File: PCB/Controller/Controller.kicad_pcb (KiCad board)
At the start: 2 copper layers, 100 x 90 mm, 25 parts, among them J1 Conn_01x03, J2 Conn_01x02, J3 Conn_01x08, J4 Conn_01x06, Q1 MJD6039, Q2 MJD6039, Q3 MJD6039, Q4 MJD6039, Q5 MJD6039, Q6 MJD6039, Q7 MJD6039, U1 ESP8266-01/ESP-01, U2 EK-TM4C123GXL

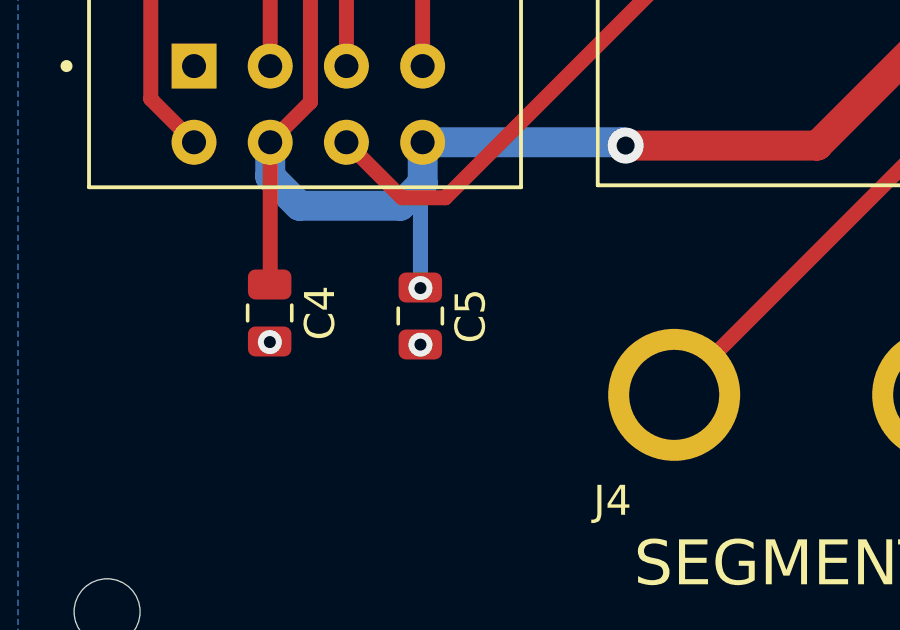
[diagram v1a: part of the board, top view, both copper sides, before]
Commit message: latest update of pcbs
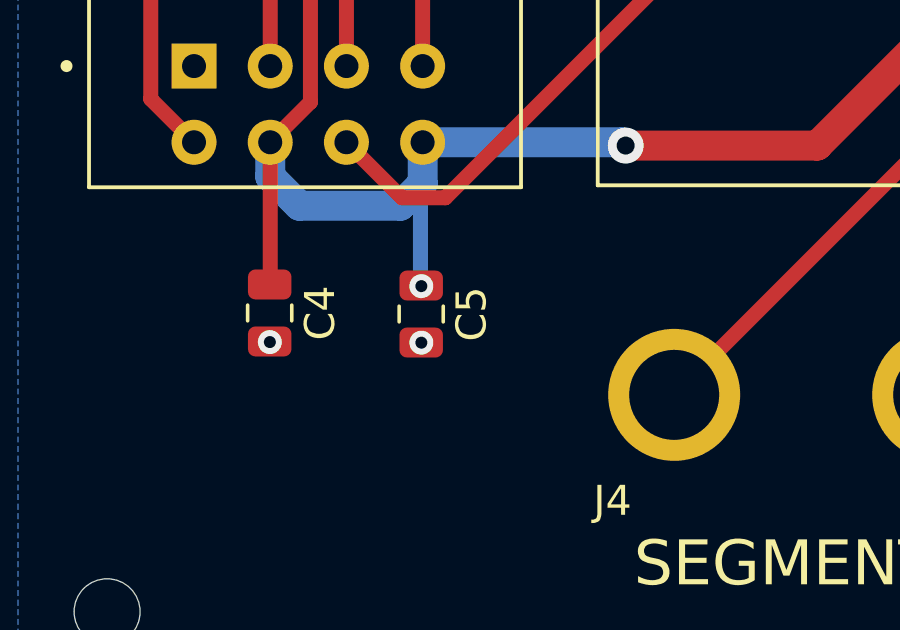
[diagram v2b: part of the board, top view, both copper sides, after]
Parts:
- moved C5 0.07 mm to (30.5, 90.1)
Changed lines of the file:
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@@
   )
   (footprint "Capacitor_SMD:C_0805_2012Metric" (layer "F.Cu")
-    (at 30.44 90.14 -90)
+    (at 30.47 90.075 -90)
     (descr "Capacitor SMD 0805 (2012 Metric), square (rectangular) end terminal, IPC_7351 nominal, (Body size source: IPC-SM-782 page 76, https://www.pcb-3d.com/wordpress/wp-content/uploads/ipc-sm-782a_amendment_1_and_2.pdf, https://docs.google.com/spreadsheets/d/1BsfQQcO9C6DZCsRaXUlFlo91Tg2WpOkGARC1WS5S8t0/edit?usp=sharing), generated with kicad-footprint-generator")
     (tags "capacitor")
@@
   (segment (start 27.315 50.225) (end 38.895 50.225) (width 1) (layer "F.Cu") (net 1))
   (via (at 47.705 80.43) (size 1.2) (drill 0.6) (layers "F.Cu" "B.Cu") (net 1))
-  (via (at 30.445 89.21) (size 0.8) (drill 0.4) (layers "F.Cu" "B.Cu") (net 1))
+  (via (at 30.475 89.145) (size 0.8) (drill 0.4) (layers "F.Cu" "B.Cu") (net 1))
   (via (at 37.285 84.46) (size 1.2) (drill 0.6) (layers "F.Cu" "B.Cu") (net 1))
   (segment (start 26.41 86.465) (end 25.4375 85.4925) (width 1) (layer "B.Cu") (net 1))
@@
   (segment (start 47.7025 80.4325) (end 47.705 80.43) (width 1) (layer "B.Cu") (net 1))
   (via (at 29.92 58.905) (size 0.8) (drill 0.4) (layers "F.Cu" "B.Cu") (net 2))
-  (via (at 30.445 91.095) (size 0.8) (drill 0.4) (layers "F.Cu" "B.Cu") (net 2))
+  (via (at 30.475 91.03) (size 0.8) (drill 0.4) (layers "F.Cu" "B.Cu") (net 2))
   (via (at 29.87 62.66) (size 0.8) (drill 0.4) (layers "F.Cu" "B.Cu") (net 2))
   (via (at 25.425 91.01) (size 0.8) (drill 0.4) (layers "F.Cu" "B.Cu") (net 2))
